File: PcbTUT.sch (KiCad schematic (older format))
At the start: 24 parts, among them SW1 SW_Push, U1 ATmega32U4-AU, Y1 16Mhz

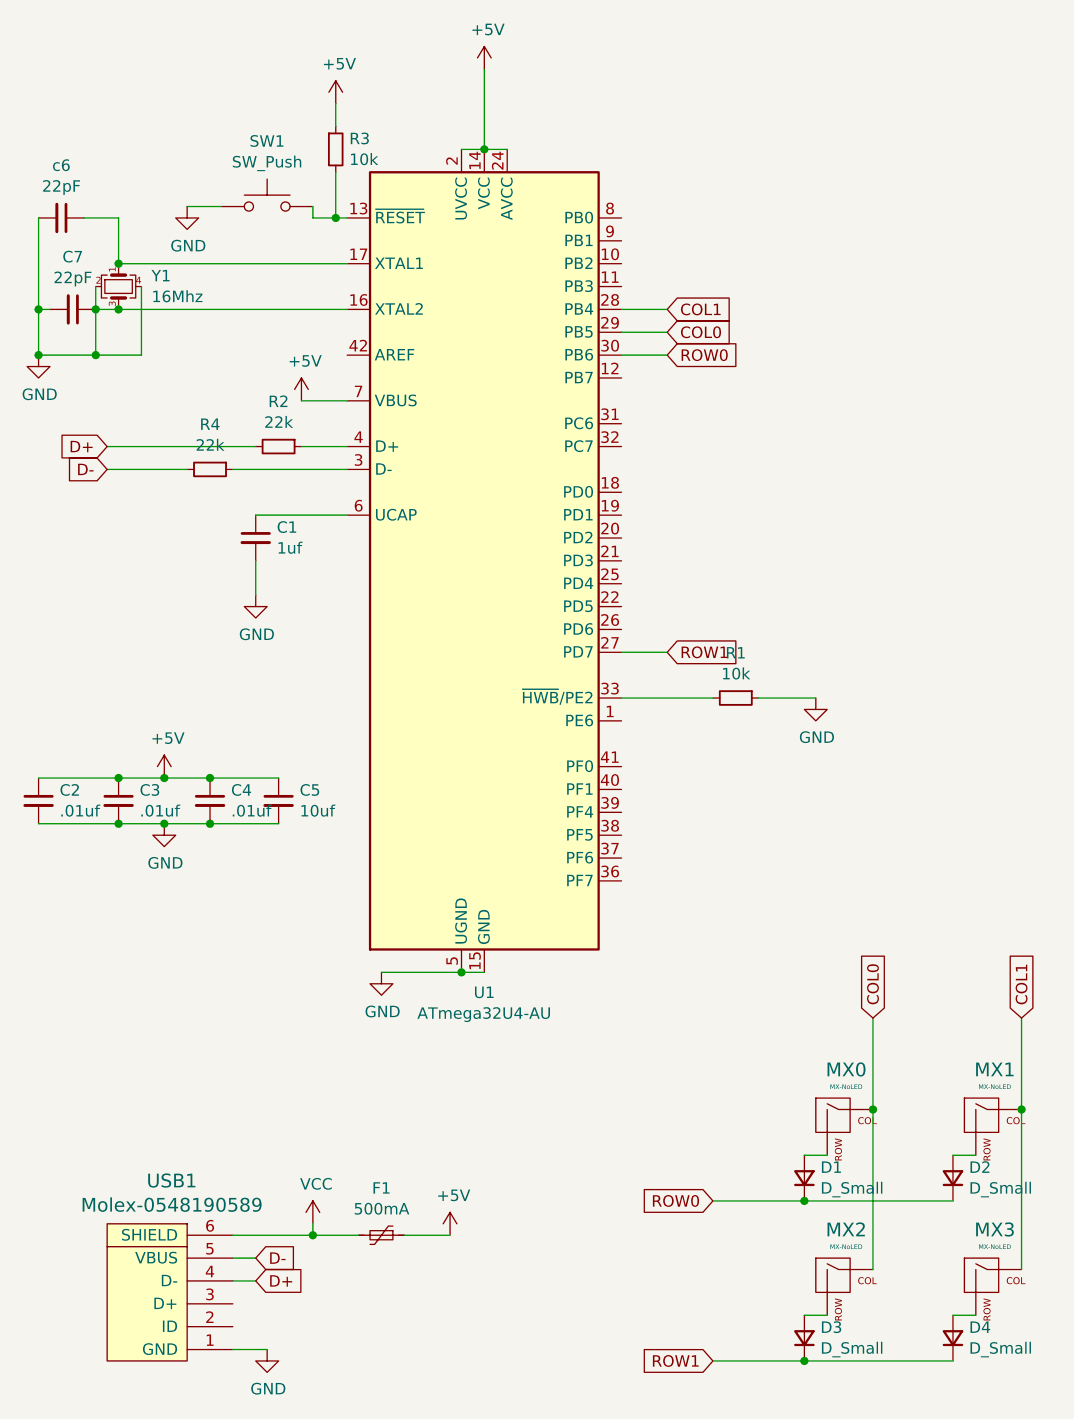
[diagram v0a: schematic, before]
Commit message: route pcb
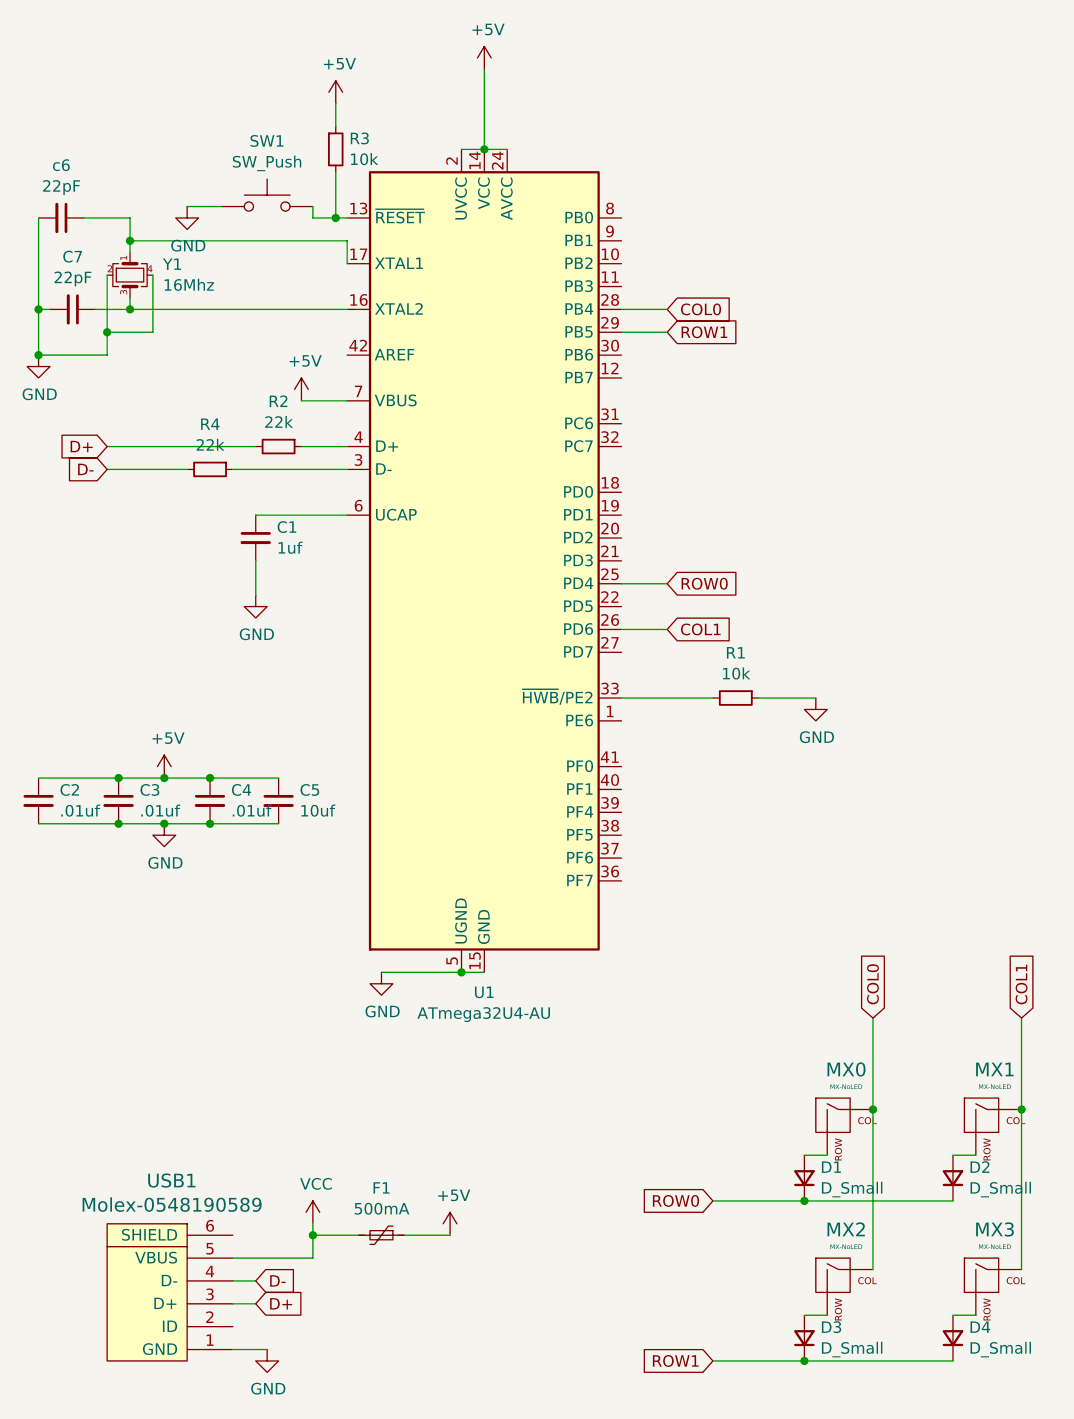
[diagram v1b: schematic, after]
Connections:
- net COL0: now also U1.28 (PB4); no longer U1.29 (PB5)
- net COL1: now also U1.26 (PD6); no longer U1.28 (PB4)
- net D+: now also USB1.3 (D+); no longer USB1.4 (D-)
- net D-: now also USB1.4 (D-); no longer USB1.5 (VBUS)
- net GND: no longer C7.1, U1.16 (XTAL2), Y1.3
- net ROW0: now also U1.25 (PD4); no longer U1.30 (PB6)
- net ROW1: now also U1.29 (PB5); no longer U1.27 (PD7)
- net VCC: now also USB1.5 (VBUS); no longer USB1.6 (SHIELD)
- new net: C7.1, U1.16 (XTAL2), Y1.3
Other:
- moved on the sheet: Y1
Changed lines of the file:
@@
 $EndDescr
-$Comp
-L MCU_Microchip_ATmega:ATmega32U4-AU U1
-U 1 1 5EF7BB6E
-P 2500 3200
-F 0 "U1" H 2500 1311 50  0000 C CNN
-F 1 "ATmega32U4-AU" H 2500 1220 50  0000 C CNN
-F 2 "Package_QFP:TQFP-44_10x10mm_P0.8mm" H 2500 3200 50  0001 C CIN
-F 3 "http://ww1.microchip.com/downloads/en/DeviceDoc/Atmel-7766-8-bit-AVR-ATmega16U4-32U4_Datasheet.pdf" H 2500 3200 50  0001 C CNN
-	1    2500 3200
-	1    0    0    -1
-$EndComp
 $Comp
 L power:+5V #PWR0101
@@
 	2400 1400 2500 1400
 Connection ~ 2500 1400
-Wire Wire Line
-	2500 1400 2500 1050
 $Comp
 L power:GND #PWR0102
@@
 	1    0    0    -1
 $EndComp
-Wire Wire Line
-	2500 5000 2400 5000
-Wire Wire Line
-	2400 5000 2050 5000
-Connection ~ 2400 5000
 $Comp
 L Device:R_Small R1
@@
 	1    0    0    -1
 $EndComp
-Wire Wire Line
-	3100 3800 3500 3800
-Wire Wire Line
-	3700 3800 3950 3800
 $Comp
 L Device:R_Small R2
@@
 	1900 2500 1700 2500
 $Comp
-L Device:Crystal_GND24_Small Y1
-U 1 1 5EF9C258
-P 900 2000
-F 0 "Y1" V 854 2144 50  0000 L CNN
-F 1 "16Mhz" V 945 2144 50  0000 L CNN
-F 2 "Crystal:Crystal_SMD_3225-4Pin_3.2x2.5mm" H 900 2000 50  0001 C CNN
-F 3 "~" H 900 2000 50  0001 C CNN
-	1    900  2000
-	0    1    1    0
-$EndComp
-Wire Wire Line
-	1900 1900 900  1900
-Wire Wire Line
-	1900 2100 900  2100
-$Comp
 L power:GND #PWR0108
 U 1 1 5EFA06B3
@@
 	0    1    1    0
 $EndComp
-Wire Wire Line
-	900  1900 900  1700
-Wire Wire Line
-	900  1700 750  1700
-Connection ~ 900  1900
-Wire Wire Line
-	550  1700 550  2100
-Wire Wire Line
-	600  2100 550  2100
-Connection ~ 550  2100
-Wire Wire Line
-	550  2100 550  2300
-Wire Wire Line
-	800  2100 900  2100
-Connection ~ 900  2100
-Wire Wire Line
-	800  2000 800  2100
-Wire Wire Line
-	800  2300 550  2300
-Connection ~ 800  2100
-Wire Wire Line
-	800  2100 800  2300
-Connection ~ 550  2300
-Wire Wire Line
-	1000 2000 1000 2300
-Wire Wire Line
-	1000 2300 800  2300
-Connection ~ 800  2300
 $Comp
 L power:GND #PWR0109
@@
 Wire Wire Line
 	1750 6100 1750 6150
-Connection ~ 1750 6150
-Wire Wire Line
-	1750 6150 1400 6150
 Wire Wire Line
 	2150 6150 2350 6150
-Text GLabel 1500 6250 2    50   Input ~ 0
+Text GLabel 1500 6350 2    50   Input ~ 0
 D-
-Text GLabel 1500 6350 2    50   Input ~ 0
+Text GLabel 1500 6450 2    50   Input ~ 0
 D+
 Wire Wire Line
 	1500 6350 1400 6350
-Wire Wire Line
-	1400 6250 1500 6250
 $Comp
 L MX_Alps_Hybrid:MX-NoLED MX0
@@
 Text GLabel 3500 6700 0    50   Input ~ 0
 ROW1
+Text GLabel 3300 2100 2    50   Input ~ 0
+COL0
+Text GLabel 3300 3500 2    50   Input ~ 0
+COL1
+Wire Wire Line
+	3300 2100 3100 2100
 Text GLabel 3300 2200 2    50   Input ~ 0
-COL0
-Text GLabel 3300 2100 2    50   Input ~ 0
-COL1
-Wire Wire Line
-	3300 2100 3100 2100
+ROW1
+Wire Wire Line
+	550  1700 550  2100
+Wire Wire Line
+	950  2100 1900 2100
+Wire Wire Line
+	950  2050 950  2100
+$Comp
+L Device:Crystal_GND24_Small Y1
+U 1 1 5EF9C258
+P 950 1950
+F 0 "Y1" V 904 2094 50  0000 L CNN
+F 1 "16Mhz" V 995 2094 50  0000 L CNN
+F 2 "Crystal:Crystal_SMD_3225-4Pin_3.2x2.5mm" H 950 1950 50  0001 C CNN
+F 3 "~" H 950 1950 50  0001 C CNN
+	1    950  1950
+	0    1    1    0
+$EndComp
+Wire Wire Line
+	1900 1800 950  1800
+Wire Wire Line
+	950  1800 950  1850
+Wire Wire Line
+	600  2100 550  2100
+Connection ~ 550  2100
+Wire Wire Line
+	550  2100 550  2300
+Wire Wire Line
+	850  2300 550  2300
+Wire Wire Line
+	850  1950 850  2200
+Connection ~ 550  2300
+Wire Wire Line
+	1050 1950 1050 2200
+Wire Wire Line
+	1050 2200 850  2200
+Connection ~ 850  2200
+Wire Wire Line
+	850  2200 850  2300
+Wire Wire Line
+	800  2100 950  2100
+Connection ~ 950  2100
+Wire Wire Line
+	950  1800 950  1700
+Wire Wire Line
+	950  1700 750  1700
+Connection ~ 950  1800
+Connection ~ 2400 5000
+Wire Wire Line
+	2400 5000 2050 5000
+Wire Wire Line
+	2500 5000 2400 5000
+Wire Wire Line
+	2500 1400 2500 1050
+Wire Wire Line
+	1900 1900 1900 1800
+$Comp
+L MCU_Microchip_ATmega:ATmega32U4-AU U1
+U 1 1 5EF7BB6E
+P 2500 3200
+F 0 "U1" H 2500 1311 50  0000 C CNN
+F 1 "ATmega32U4-AU" H 2500 1220 50  0000 C CNN
+F 2 "Package_QFP:TQFP-44_10x10mm_P0.8mm" H 2500 3200 50  0001 C CIN
+F 3 "http://ww1.microchip.com/downloads/en/DeviceDoc/Atmel-7766-8-bit-AVR-ATmega16U4-32U4_Datasheet.pdf" H 2500 3200 50  0001 C CNN
+	1    2500 3200
+	1    0    0    -1
+$EndComp
+Wire Wire Line
+	3300 3300 3100 3300
+Text GLabel 3300 3300 2    50   Input ~ 0
+ROW0
+Wire Wire Line
+	3700 3800 3950 3800
+Wire Wire Line
+	3100 3800 3500 3800
+Wire Wire Line
+	3100 3500 3300 3500
+Wire Wire Line
+	1500 6450 1400 6450
+Wire Wire Line
+	1750 6150 1750 6250
+Wire Wire Line
+	1750 6250 1400 6250
+Connection ~ 1750 6150
 Wire Wire Line
 	3300 2200 3100 2200
-Text GLabel 3300 2300 2    50   Input ~ 0
-ROW0
-Text GLabel 3300 3600 2    50   Input ~ 0
-ROW1
-Wire Wire Line
-	3100 3600 3300 3600
-Wire Wire Line
-	3300 2300 3100 2300
 $EndSCHEMATC
